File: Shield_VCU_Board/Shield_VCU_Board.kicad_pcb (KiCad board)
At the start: 2 copper layers, 250.5 x 110 mm, 148 parts, among them J1 Conn_02x08_Odd_Even, J10 Main_Supply, J11 Conn_01x40_Socket, J13 Conn_Molex_TouchPanel, J14 CAN_OUT, J15 Conn_01x04_Socket, J2 Conn_02x10_Odd_Even, J3/1 NXP3, J4 Conn_02x08_Odd_Even, J5 Conn_02x10_Odd_Even, J6 Conn_02x10_Odd_Even, J7 Button_Activation_Logic, J8 Conn_ToSpeaker, U1 AS1115-BSST, U10 TPS61165DBV, U2 SN74LVC1G125DBV, U3 MC74HC14A, U4 TPA6205A1, U5 TLV76133DCY, U6 TLV76150DCY, U7 FT812, U8 TLV76133DCY, U9 TLV76133DCY, Y2 SG-210STF

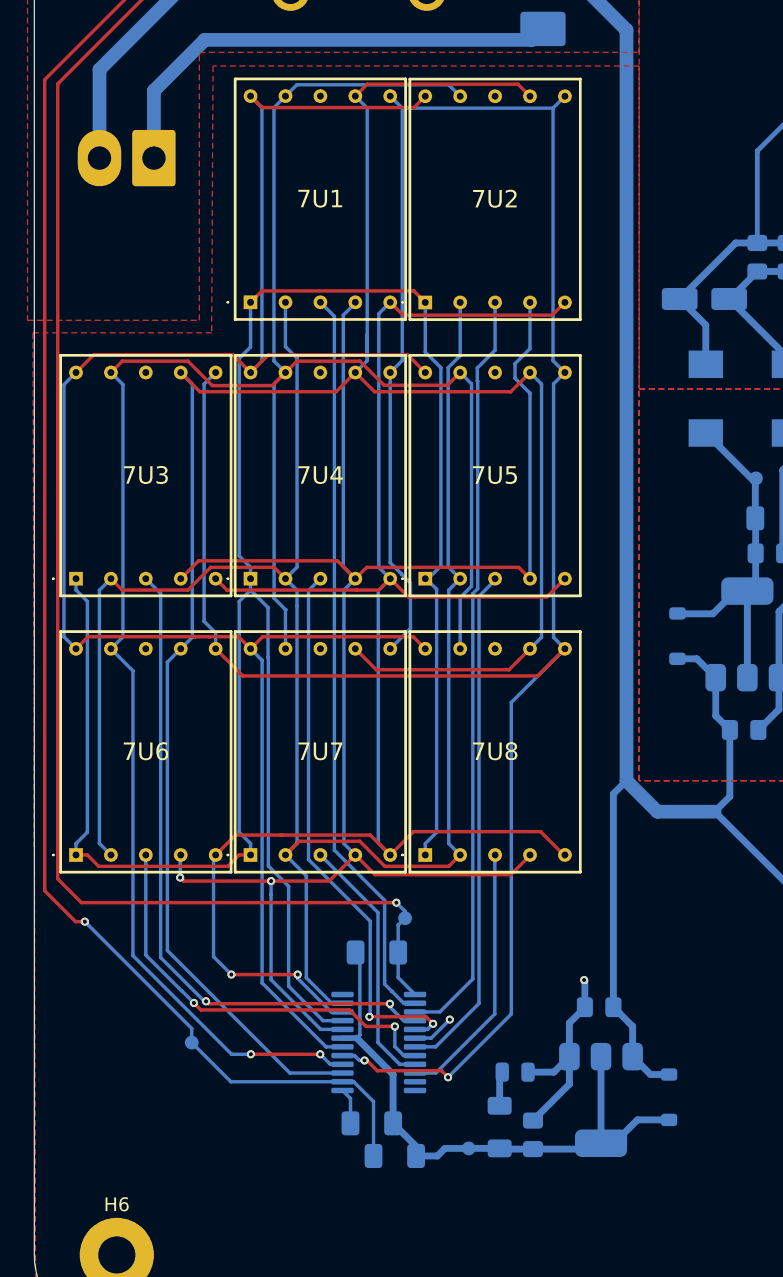
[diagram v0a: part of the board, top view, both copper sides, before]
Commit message: Required_corr_0.4
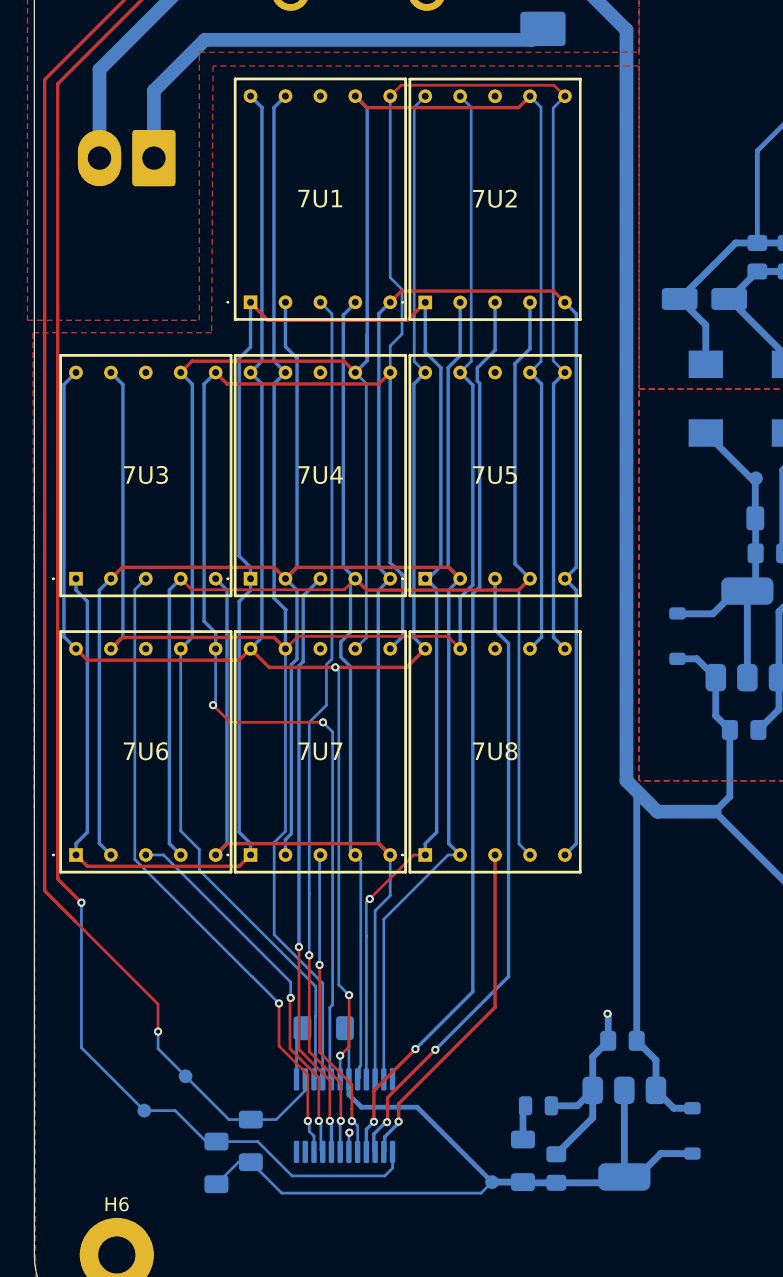
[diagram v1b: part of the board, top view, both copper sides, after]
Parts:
- moved SDA7 23.6 mm to (33.0, 137.5), turned to 90 degrees
- moved R55 19.2 mm to (38.2, 141.3), turned to 90 degrees
- moved R56 10.5 mm to (40.8, 139.7), turned to 90 degrees
- moved RSET1 7.76 mm to (46.1, 131.5)
- moved U1 5.87 mm to (47.6, 137.9), turned to 90 degrees
- moved C31 2.98 mm to (67.8, 132.4)
- moved C32 2.98 mm to (63.0, 141.7)
- moved U8 2.98 mm to (67.9, 139.2)
- moved D12 2.98 mm to (61.7, 137.2)
- moved R52 2.98 mm to (60.5, 141.2)
- moved D9 2.98 mm to (72.9, 139.0)
- moved SEGV3.3 2.98 mm to (58.3, 142.7)
- moved SCL7 2.49 mm to (36.0, 135.0), turned to 90 degrees
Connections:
- 7U1 pad 3: Net-(U1-DIG0) -> Net-(U1-DIG4)
- 7U2 pad 3: Net-(U1-DIG1) -> Net-(U1-DIG2)
- 7U3 pad 3: Net-(U1-DIG2) -> Net-(U1-DIG7)
- 7U4 pad 3: Net-(U1-DIG3) -> Net-(U1-DIG5)
- 7U5 pad 3: Net-(U1-DIG4) -> Net-(U1-DIG1)
- 7U6 pad 3: Net-(U1-DIG5) -> Net-(U1-DIG6)
- 7U7 pad 3: Net-(U1-DIG6) -> Net-(U1-DIG3)
- 7U8 pad 3: Net-(U1-DIG7) -> Net-(U1-DIG0)
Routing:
- net Net-(U1-DIG0): track 54.3 -> 25.0 mm, vias 0 -> 1
- net Net-(U1-DIG7): track 19.2 -> 47.4 mm, vias 0 -> 2
- net Net-(U1-DIG4): track 37.3 -> 63.8 mm, vias 0 -> 2
- net Net-(7U1-G): track 141.9 -> 161.8 mm, vias 0 -> 3
- net Net-(7U1-DP): track 129.1 -> 147.8 mm, vias 2 -> 0
- net 3V3_7seg: track 43.7 -> 61.8 mm
- net Net-(U1-DIG3): track 40.4 -> 22.8 mm
- net Net-(U1-DIG2): track 48.6 -> 65.8 mm
- net Net-(7U1-E): track 166.1 -> 150.1 mm, vias 0 -> 1
- net Net-(7U1-B): track 185.6 -> 169.9 mm
- net Net-(7U1-C): track 132.9 -> 147.8 mm, vias 2 -> 0
- net Net-(U1-DIG5): track 30.9 -> 43.3 mm
- net Net-(7U1-A): track 158.0 -> 167.8 mm
- net Net-(U1-DIG6): track 18.7 -> 27.7 mm, vias 0 -> 2
- net Net-(U1-DIG1): track 55.1 -> 46.4 mm, vias 0 -> 2
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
